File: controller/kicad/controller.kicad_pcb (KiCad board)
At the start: 2 copper layers, 90 x 80 mm, 22 parts, among them J1 pcie_98, U1 ESD5344D, U10 ESD5344D, U11 WeAct_STM32H750_Module, U12 ESD5344D, U13 ESD5344D, U14 ESD5344D, U15 ESD5344D, U16 ESD5344D, U17 ESD5344D, U18 ESD5344D, U19 ESD5344D, U2 ESD5344D, U20 ESD5344D, U21 ESD5344D, U3 ESD5344D, U4 ESD5344D, U5 ESD5344D, U6 ESD5344D, U7 ESD5344D, U8 ESD5344D, U9 ESD5344D

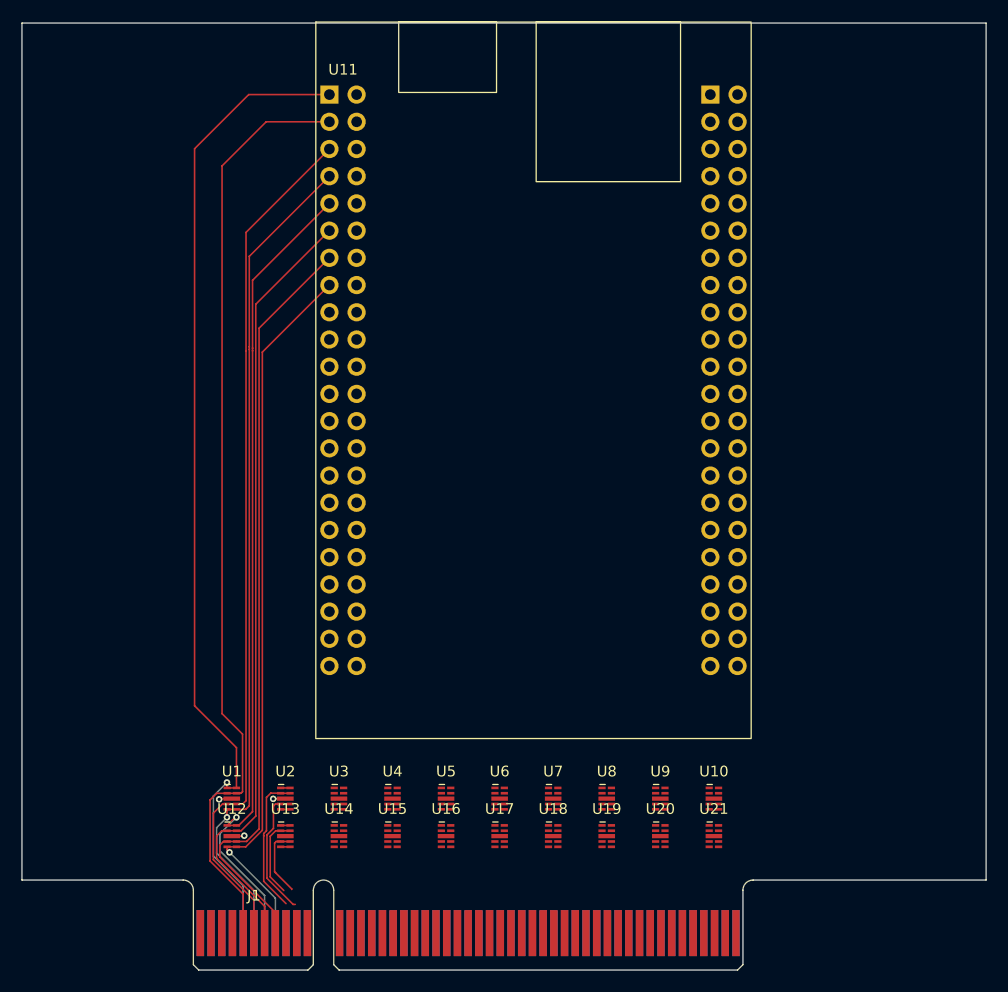
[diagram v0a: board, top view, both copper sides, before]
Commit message: Work in progress. Rouging the MCU signals.
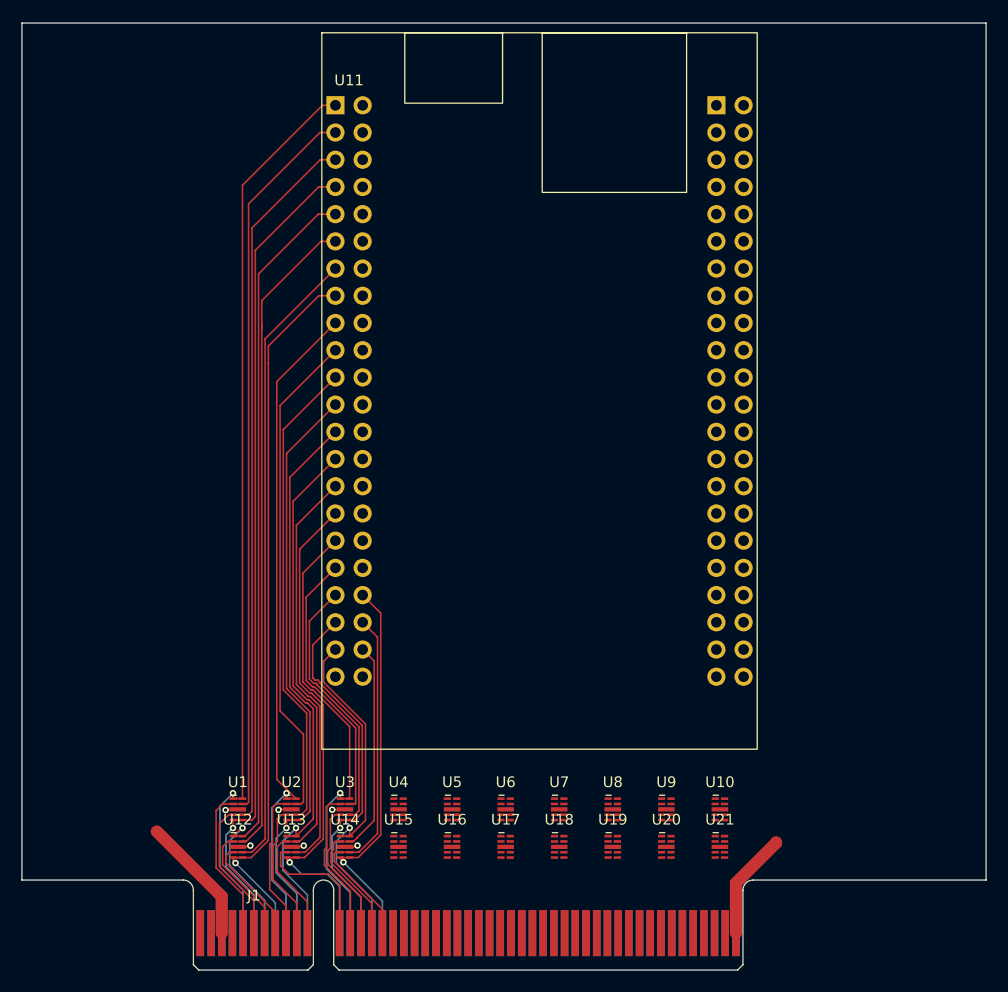
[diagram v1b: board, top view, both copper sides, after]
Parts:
- moved U1 1.15 mm to (62.0, 45.0)
- moved U10 1.15 mm to (107.0, 45.0)
- moved U11 1.15 mm to (90.2, 5.95)
- moved U12 1.15 mm to (62.0, 48.5)
- moved U13 1.15 mm to (67.0, 48.5)
- moved U14 1.15 mm to (72.0, 48.5)
- moved U15 1.15 mm to (77.0, 48.5)
- moved U16 1.15 mm to (82.0, 48.5)
- moved U17 1.15 mm to (87.0, 48.5)
- moved U18 1.15 mm to (92.0, 48.5)
- moved U19 1.15 mm to (97.0, 48.5)
- moved U2 1.15 mm to (67.0, 45.0)
- moved U20 1.15 mm to (102.0, 48.5)
- moved U21 1.15 mm to (107.0, 48.5)
- moved U3 1.15 mm to (72.0, 45.0)
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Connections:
- J1 pad A10: /PB1 -> /PC11
- J1 pad A11: /PE7 -> /PD0
- J1 pad A12: /PE13 -> /PD6
- J1 pad A13: /PB15 -> /PB3
- J1 pad A14: /A -> /PB9
- J1 pad A15: /A -> /PE1
- J1 pad A16: /A -> /PB6
- J1 pad A9: /PC5 -> /PA9
- J1 pad B10: /PE9 -> /PA15
- J1 pad B11: /PE11 -> /PD2
- J1 pad B12: /PB11 -> /PD4
- J1 pad B13: /B -> /PB5
- J1 pad B14: /B -> /PB7
- J1 pad B15: /B -> /PE0
- J1 pad B16: /B -> /PB8
- J1 pad B9: /PB3 -> /PA11
- U10 pad 1: unconnected-(U10-Pad1) -> /X
- U10 pad 2: unconnected-(U10-Pad2) -> /X
- U10 pad 4: unconnected-(U10-Pad4) -> /X
- U10 pad 5: unconnected-(U10-Pad5) -> /X
- U14 pad 1: unconnected-(U14-Pad1) -> /PE1
- U14 pad 2: unconnected-(U14-Pad2) -> /PE0
- U14 pad 4: unconnected-(U14-Pad4) -> /PB8
- U14 pad 5: unconnected-(U14-Pad5) -> /PB6
- U15 pad 1: unconnected-(U15-Pad1) -> /X
- U15 pad 2: unconnected-(U15-Pad2) -> /X
- U15 pad 4: unconnected-(U15-Pad4) -> /X
- U15 pad 5: unconnected-(U15-Pad5) -> /X
- U16 pad 1: unconnected-(U16-Pad1) -> /X
- U16 pad 2: unconnected-(U16-Pad2) -> /X
- U16 pad 4: unconnected-(U16-Pad4) -> /X
- U16 pad 5: unconnected-(U16-Pad5) -> /X
- U17 pad 1: unconnected-(U17-Pad1) -> /X
- U17 pad 2: unconnected-(U17-Pad2) -> /X
- U17 pad 4: unconnected-(U17-Pad4) -> /X
- U17 pad 5: unconnected-(U17-Pad5) -> /X
- U18 pad 1: unconnected-(U18-Pad1) -> /X
- U18 pad 2: unconnected-(U18-Pad2) -> /X
- U18 pad 4: unconnected-(U18-Pad4) -> /X
- U18 pad 5: unconnected-(U18-Pad5) -> /X
- U19 pad 1: unconnected-(U19-Pad1) -> /X
- U19 pad 2: unconnected-(U19-Pad2) -> /X
- U19 pad 4: unconnected-(U19-Pad4) -> /X
- U19 pad 5: unconnected-(U19-Pad5) -> /X
- U20 pad 1: unconnected-(U20-Pad1) -> /X
- U20 pad 2: unconnected-(U20-Pad2) -> /X
- U20 pad 4: unconnected-(U20-Pad4) -> /X
- U20 pad 5: unconnected-(U20-Pad5) -> /X
- U21 pad 1: unconnected-(U21-Pad1) -> /X
- U21 pad 2: unconnected-(U21-Pad2) -> /X
- U21 pad 4: unconnected-(U21-Pad4) -> /X
- U21 pad 5: unconnected-(U21-Pad5) -> /X
- U3 pad 1: unconnected-(U3-Pad1) -> /PB3
- U3 pad 2: unconnected-(U3-Pad2) -> /PB5
- U3 pad 4: unconnected-(U3-Pad4) -> /PB7
- U3 pad 5: unconnected-(U3-Pad5) -> /PB9
- U4 pad 1: unconnected-(U4-Pad1) -> /X
- U4 pad 2: unconnected-(U4-Pad2) -> /X
- U4 pad 4: unconnected-(U4-Pad4) -> /X
- U4 pad 5: unconnected-(U4-Pad5) -> /X
- U5 pad 1: unconnected-(U5-Pad1) -> /X
- U5 pad 2: unconnected-(U5-Pad2) -> /X
- U5 pad 4: unconnected-(U5-Pad4) -> /X
- U5 pad 5: unconnected-(U5-Pad5) -> /X
- U6 pad 1: unconnected-(U6-Pad1) -> /X
- U6 pad 2: unconnected-(U6-Pad2) -> /X
- U6 pad 4: unconnected-(U6-Pad4) -> /X
- U6 pad 5: unconnected-(U6-Pad5) -> /X
- U7 pad 1: unconnected-(U7-Pad1) -> /X
- U7 pad 2: unconnected-(U7-Pad2) -> /X
- U7 pad 4: unconnected-(U7-Pad4) -> /X
- U7 pad 5: unconnected-(U7-Pad5) -> /X
- U8 pad 1: unconnected-(U8-Pad1) -> /X
- U8 pad 2: unconnected-(U8-Pad2) -> /X
- U8 pad 4: unconnected-(U8-Pad4) -> /X
- U8 pad 5: unconnected-(U8-Pad5) -> /X
- U9 pad 1: unconnected-(U9-Pad1) -> /X
- U9 pad 2: unconnected-(U9-Pad2) -> /X
- U9 pad 4: unconnected-(U9-Pad4) -> /X
- U9 pad 5: unconnected-(U9-Pad5) -> /X
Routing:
- net /PA9: track 0.88 -> 63.0 mm, vias 0 -> 1
- net /PC11: track 0.88 -> 55.0 mm, vias 0 -> 1
- net /PD0: track 0.88 -> 54.1 mm, vias 0 -> 1
- net /PA11: track 13.3 -> 60.8 mm
- net /PD6: track 0.88 -> 47.4 mm, vias 0 -> 1
- net /PA15: track 12.3 -> 58.1 mm
- net /PD4: track 6.49 -> 51.5 mm
- net /PB3: track 0.00 -> 43.2 mm, vias 0 -> 1
- net /PD2: track 7.66 -> 50.5 mm
- net /PB5: track 0.00 -> 40.8 mm
- net /PB7: track 0.00 -> 38.2 mm
- net /PB6: track 0.00 -> 36.4 mm, vias 0 -> 1
- net /PB9: track 0.00 -> 35.1 mm, vias 0 -> 1
- net /PB8: track 0.00 -> 34.4 mm
- net /PE1: track 0.00 -> 33.5 mm, vias 0 -> 1
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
